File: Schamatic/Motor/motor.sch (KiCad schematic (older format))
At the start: 45 parts, among them J1 CONN_02X05, J11 V, J12 U, J13 W, J3 RS485, J6 12, J9 GND, Q1 PSMN3R3-40YS, Q2 PSMN3R3-40YS, Q3 PSMN3R3-40YS, Q4 PSMN3R3-40YS, Q5 PSMN3R3-40YS, Q6 PSMN3R3-40YS, U1 STSPIN32F0, U2 LTC2876, U3 MA700, U4 A1335, Y1 8Mhz

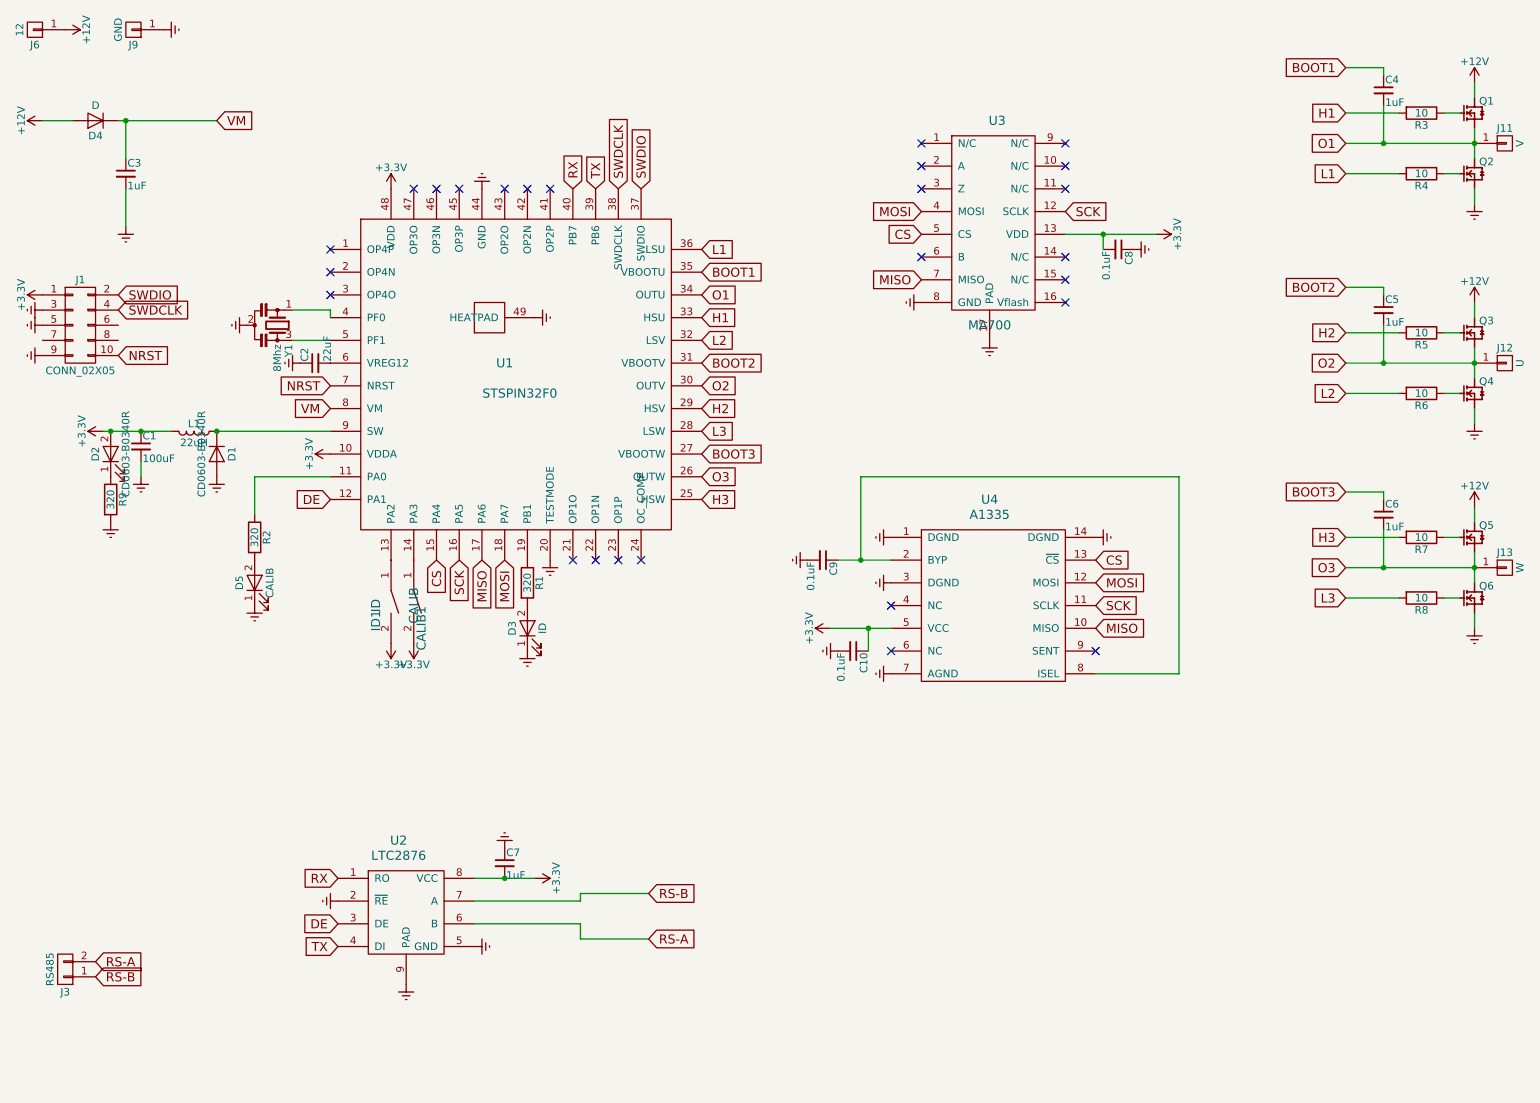
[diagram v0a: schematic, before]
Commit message: high voltage controller
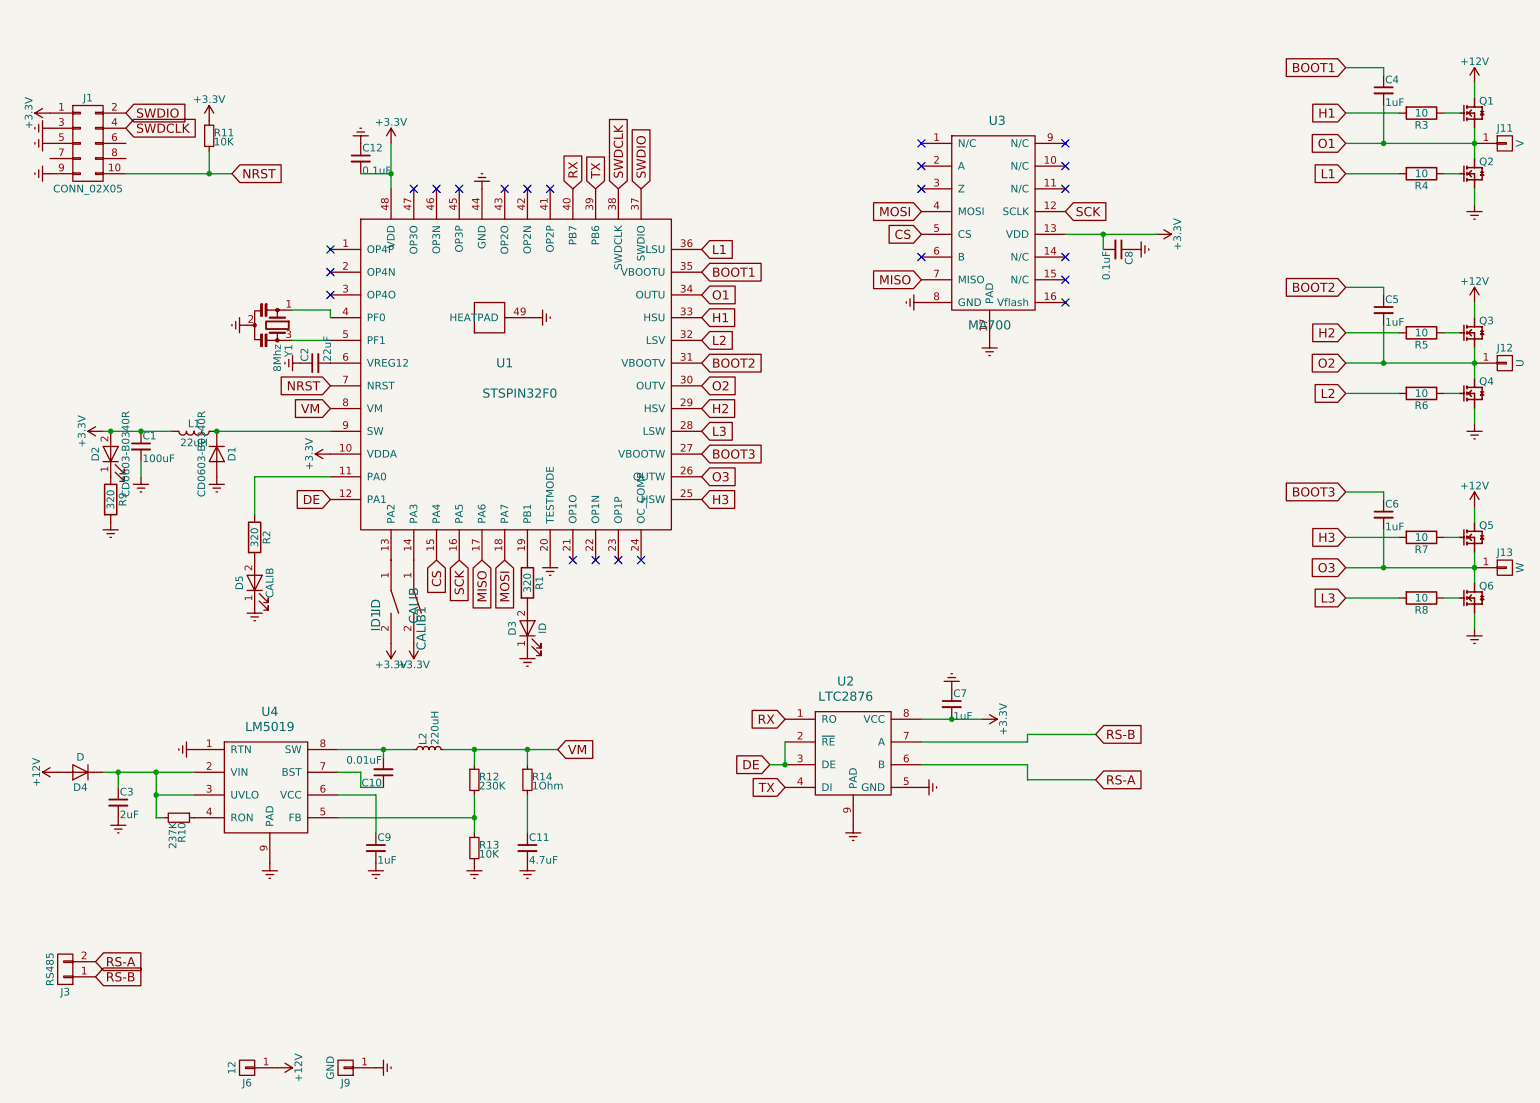
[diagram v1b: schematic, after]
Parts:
- removed U4: A1335, Housings_SSOP:TSSOP-14_4.4x5mm_Pitch0.65mm, symbol A1335
- added C11: 4.7uF, Capacitors_SMD:C_1206, symbol C_Small
- added C12: 0.1uF, Capacitors_SMD:C_0603, symbol C_Small
- added L2: 220uH, Inductors_SMD:L_1210, symbol L_Small
- added R10: 237K, Capacitors_SMD:C_0603, symbol R_Small
- added R11, R13: 10K, Capacitors_SMD:C_0603, symbol R_Small
- added R12: 230K, Capacitors_SMD:C_0603, symbol R_Small
- added R14: 1Ohm, Capacitors_SMD:C_0603, symbol R_Small
- added U4: LM5019, Housings_DFN_QFN:DFN-8-1EP_4x4mm_Pitch0.8mm, symbol LM5019
- C1: footprint Capacitors_SMD:C_0805 -> Capacitors_SMD:C_1210
- C10: value 0.1uF -> 0.01uF
- C3: value 1uF -> 2uF; footprint Capacitors_SMD:C_1206 -> Capacitors_SMD:C_1210
- C9: value 0.1uF -> 1uF
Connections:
- net +3V3: now also C12.2, R11.1; no longer C10.1
- net DE: now also U2.2 (~RE)
- net Earth: now also C11.2, C12.1, R13.2, U4.1 (RTN), U4.9 (PAD); no longer C10.2, U2.2 (~RE)
- net NRST: now also R11.2
- net VM: now also L2.2, R12.1, R14.1; no longer C3.1, D4.1 (K)
- net at C9.1: now also U4.6 (VCC)
- new net: C3.1, D4.1 (K), R10.2, U4.2 (VIN), U4.3 (UVLO)
- new net: R10.1, U4.4 (RON)
- new net: R12.2, R13.1, U4.5 (FB)
- new net: C10.1, U4.7 (BST)
- new net: C10.2, L2.1, U4.8 (SW)
- new net: C11.1, R14.2
- no-connect marks 26 -> 23
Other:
- moved on the sheet: C3, C7, D4, J1, J6, J9, U2
